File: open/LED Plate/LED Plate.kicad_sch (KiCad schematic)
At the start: 5 parts, among them J1 Conn_01x02

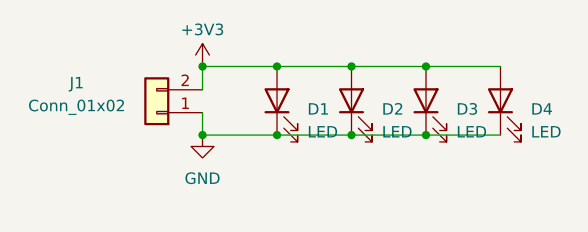
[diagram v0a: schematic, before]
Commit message: L1- 5050 LED
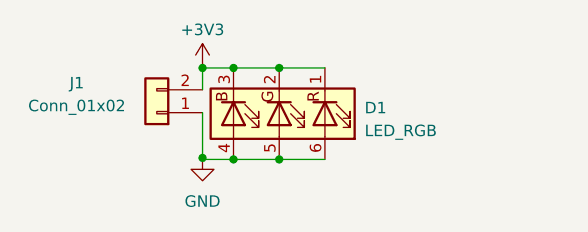
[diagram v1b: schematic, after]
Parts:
- removed D1, D2, D3, D4: LED, 2024l1:LED-3528, symbol Device:LED
- added D1: LED_RGB, LED_SMD:LED_RGB_5050-6, symbol Device:LED_RGB
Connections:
- net +3V3: now also D1.1 (RK), D1.2 (GK), D1.3 (BK)
- net GND: now also D1.4 (BA), D1.5 (GA), D1.6 (RA)
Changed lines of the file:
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@@
 (kicad_sch (version 20230121) (generator eeschema)
   (paper "A4")
-  (junction (at 81.3001 78.2791) (diameter 0) (color 0 0 0 0)
+  (junction (at 81.5455 70.8246) (diameter 0) (color 0 0 0 0)
   )
-  (junction (at 97.8527 70.6591) (diameter 0) (color 0 0 0 0)
+  (junction (at 81.5455 80.9846) (diameter 0) (color 0 0 0 0)
   )
-  (junction (at 89.5764 70.6591) (diameter 0) (color 0 0 0 0)
+  (junction (at 73.0238 70.8246) (diameter 0) (color 0 0 0 0)
   )
-  (junction (at 73.0238 78.2791) (diameter 0) (color 0 0 0 0)
+  (junction (at 73.0238 80.8191) (diameter 0) (color 0 0 0 0)
   )
-  (junction (at 73.0238 70.6591) (diameter 0) (color 0 0 0 0)
+  (junction (at 76.4655 80.9846) (diameter 0) (color 0 0 0 0)
   )
-  (junction (at 81.3001 70.6591) (diameter 0) (color 0 0 0 0)
+  (junction (at 76.4655 70.8246) (diameter 0) (color 0 0 0 0)
   )
-  (junction (at 97.8527 78.2791) (diameter 0) (color 0 0 0 0)
-  )
-  (junction (at 89.5764 78.2791) (diameter 0) (color 0 0 0 0)
-  )
-  (wire (pts (xy 81.3001 70.6591) (xy 73.0238 70.6591))
+  (wire (pts (xy 76.4655 70.8246) (xy 73.0238 70.8246))
     (stroke (width 0) (type default))
   )
-  (wire (pts (xy 81.3001 78.2791) (xy 89.5764 78.2791))
+  (wire (pts (xy 81.5455 70.8246) (xy 86.6255 70.8246))
     (stroke (width 0) (type default))
   )
-  (wire (pts (xy 73.0238 78.2791) (xy 81.3001 78.2791))
+  (wire (pts (xy 73.0238 70.6591) (xy 73.0238 70.8246))
     (stroke (width 0) (type default))
   )
-  (wire (pts (xy 106.129 70.6591) (xy 97.8527 70.6591))
+  (wire (pts (xy 81.5455 80.9846) (xy 86.6255 80.9846))
     (stroke (width 0) (type default))
   )
-  (wire (pts (xy 97.8527 78.2791) (xy 106.129 78.2791))
+  (wire (pts (xy 76.4655 80.9846) (xy 81.5455 80.9846))
     (stroke (width 0) (type default))
   )
-  (wire (pts (xy 73.0238 70.6591) (xy 73.0238 73.2503))
+  (wire (pts (xy 76.4655 70.8246) (xy 81.5455 70.8246))
     (stroke (width 0) (type default))
   )
-  (wire (pts (xy 73.0238 75.7903) (xy 73.0238 78.2791))
+  (wire (pts (xy 73.0238 75.7903) (xy 73.0238 80.8191))
     (stroke (width 0) (type default))
   )
-  (wire (pts (xy 89.5764 70.6591) (xy 81.3001 70.6591))
+  (wire (pts (xy 76.4655 80.9846) (xy 73.0238 80.9846))
     (stroke (width 0) (type default))
   )
-  (wire (pts (xy 97.8527 70.6591) (xy 89.5764 70.6591))
+  (wire (pts (xy 73.0238 80.9846) (xy 73.0238 80.8191))
     (stroke (width 0) (type default))
   )
-  (wire (pts (xy 89.5764 78.2791) (xy 97.8527 78.2791))
+  (wire (pts (xy 73.0238 70.8246) (xy 73.0238 73.2503))
     (stroke (width 0) (type default))
   )
-  (symbol (lib_id "Device:LED") (at 97.8527 74.4691 90) (unit 1)
+  (symbol (lib_id "Device:LED_RGB") (at 81.5455 75.9046 270) (unit 1)
     (in_bom yes) (on_board yes) (dnp no) (fields_autoplaced)
-    (property "Reference" "D3" (at 101.2196 75.4216 90)
-      (effects (font (size 1.27 1.27)) (justify right))
+    (property "Reference" "D1" (at 91.0291 75.2696 90)
+      (effects (font (size 1.27 1.27)) (justify left))
     )
-    (property "Value" "LED" (at 101.2196 77.9616 90)
-      (effects (font (size 1.27 1.27)) (justify right))
+    (property "Value" "LED_RGB" (at 91.0291 77.8096 90)
+      (effects (font (size 1.27 1.27)) (justify left))
     )
-    (property "Footprint" "2024l1:LED-3528" (at 97.8527 74.4691 0)
+    (property "Footprint" "LED_SMD:LED_RGB_5050-6" (at 80.2755 75.9046 0)
       (effects (font (size 1.27 1.27)) hide)
     )
-    (property "Datasheet" "~" (at 97.8527 74.4691 0)
+    (property "Datasheet" "~" (at 80.2755 75.9046 0)
       (effects (font (size 1.27 1.27)) hide)
     )
     (pin "1")
     (pin "2")
-    (instances
-      (project "LED Plate"
-        (path "/fcedcb69-8dd9-4ce9-8bf8-c39f35cca66f"
-          (reference "D3") (unit 1)
-        )
-      )
-    )
-  )
-  (symbol (lib_id "Device:LED") (at 89.5764 74.4691 90) (unit 1)
-    (in_bom yes) (on_board yes) (dnp no) (fields_autoplaced)
-    (property "Reference" "D2" (at 92.9433 75.4216 90)
-      (effects (font (size 1.27 1.27)) (justify right))
-    )
-    (property "Value" "LED" (at 92.9433 77.9616 90)
-      (effects (font (size 1.27 1.27)) (justify right))
-    )
-    (property "Footprint" "2024l1:LED-3528" (at 89.5764 74.4691 0)
-      (effects (font (size 1.27 1.27)) hide)
-    )
-    (property "Datasheet" "~" (at 89.5764 74.4691 0)
-      (effects (font (size 1.27 1.27)) hide)
-    )
-    (pin "1")
-    (pin "2")
-    (instances
-      (project "LED Plate"
-        (path "/fcedcb69-8dd9-4ce9-8bf8-c39f35cca66f"
-          (reference "D2") (unit 1)
-        )
-      )
-    )
-  )
-  (symbol (lib_id "Device:LED") (at 106.129 74.4691 90) (unit 1)
-    (in_bom yes) (on_board yes) (dnp no) (fields_autoplaced)
-    (property "Reference" "D4" (at 109.4959 75.4216 90)
-      (effects (font (size 1.27 1.27)) (justify right))
-    )
-    (property "Value" "LED" (at 109.4959 77.9616 90)
-      (effects (font (size 1.27 1.27)) (justify right))
-    )
-    (property "Footprint" "2024l1:LED-3528" (at 106.129 74.4691 0)
-      (effects (font (size 1.27 1.27)) hide)
-    )
-    (property "Datasheet" "~" (at 106.129 74.4691 0)
-      (effects (font (size 1.27 1.27)) hide)
-    )
-    (pin "1")
-    (pin "2")
-    (instances
-      (project "LED Plate"
-        (path "/fcedcb69-8dd9-4ce9-8bf8-c39f35cca66f"
-          (reference "D4") (unit 1)
-        )
-      )
-    )
-  )
-  (symbol (lib_id "Device:LED") (at 81.3001 74.4691 90) (unit 1)
-    (in_bom yes) (on_board yes) (dnp no) (fields_autoplaced)
-    (property "Reference" "D1" (at 84.667 75.4216 90)
-      (effects (font (size 1.27 1.27)) (justify right))
-    )
-    (property "Value" "LED" (at 84.667 77.9616 90)
-      (effects (font (size 1.27 1.27)) (justify right))
-    )
-    (property "Footprint" "2024l1:LED-3528" (at 81.3001 74.4691 0)
-      (effects (font (size 1.27 1.27)) hide)
-    )
-    (property "Datasheet" "~" (at 81.3001 74.4691 0)
-      (effects (font (size 1.27 1.27)) hide)
-    )
-    (pin "1")
-    (pin "2")
+    (pin "3")
+    (pin "4")
+    (pin "5")
+    (pin "6")
     (instances
       (project "LED Plate"
@@
     )
   )
-  (symbol (lib_id "power:GND") (at 73.0238 78.2791 0) (unit 1)
+  (symbol (lib_id "power:GND") (at 73.0238 80.8191 0) (unit 1)
     (in_bom yes) (on_board yes) (dnp no) (fields_autoplaced)
-    (property "Reference" "#PWR02" (at 73.0238 84.6291 0)
+    (property "Reference" "#PWR02" (at 73.0238 87.1691 0)
       (effects (font (size 1.27 1.27)) hide)
     )
-    (property "Value" "GND" (at 73.0238 83.1193 0)
+    (property "Value" "GND" (at 73.0238 85.6593 0)
       (effects (font (size 1.27 1.27)))
     )
-    (property "Footprint" "" (at 73.0238 78.2791 0)
+    (property "Footprint" "" (at 73.0238 80.8191 0)
       (effects (font (size 1.27 1.27)) hide)
     )
-    (property "Datasheet" "" (at 73.0238 78.2791 0)
+    (property "Datasheet" "" (at 73.0238 80.8191 0)
       (effects (font (size 1.27 1.27)) hide)
     )
